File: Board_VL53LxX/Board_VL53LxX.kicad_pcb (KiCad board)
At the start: 2 copper layers, 20 x 16 mm, 11 parts, among them J1 Conn_01x06, U1 VL53L0X

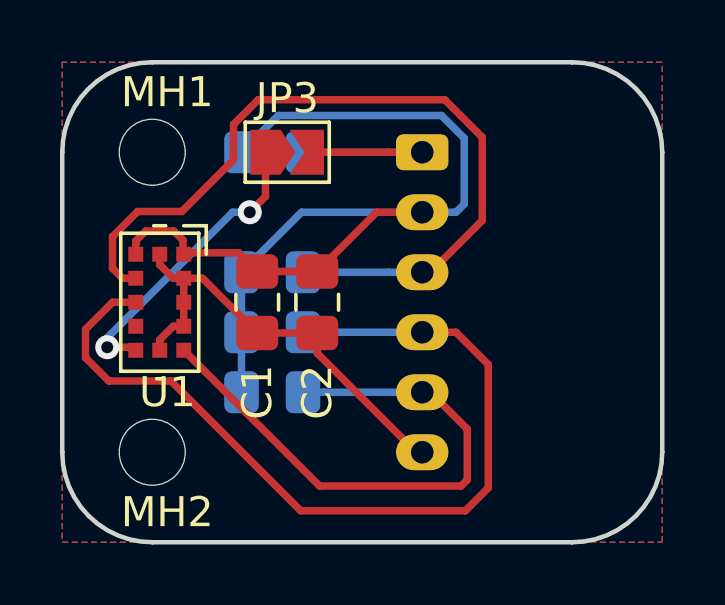
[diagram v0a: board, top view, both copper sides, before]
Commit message: update board
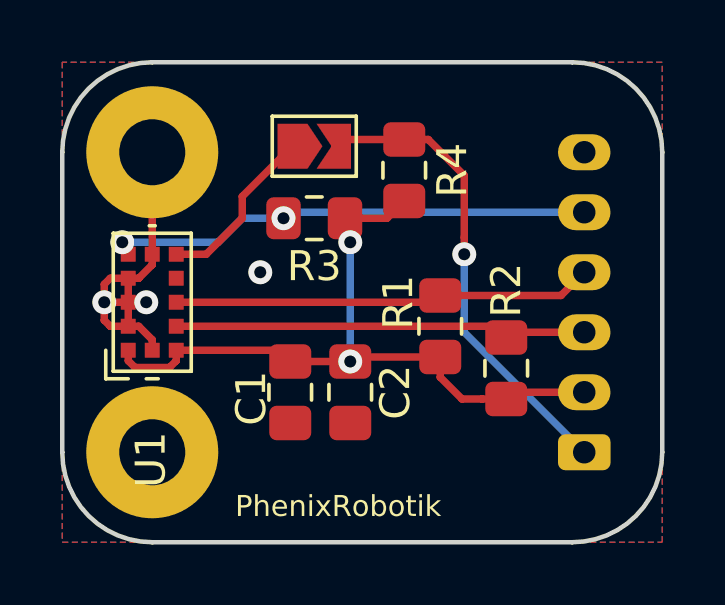
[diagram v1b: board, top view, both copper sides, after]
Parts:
- added LOGO1: Logo_Open_Hardware_Small, Symbol:OSHW-Logo2_7.3x6mm_SilkScreen, B.Cu at (107.6, 93.2)
- added LOGO2: Logo_Open_Hardware_Small, PhenixRobotik:Logo_8,5mm, B.Cu at (107.8, 84.4)
- MH1, MH2: value MountingHole -> MountingHole_Pad; footprint MountingHole:MountingHole_2.2mm_M2 -> MountingHole:MountingHole_2.2mm_M2_Pad
- R1, R2, R3, R4: moved to F.Cu
- U1: footprint PhoenixRobotik:TOF-12_4.4x2.4x1.0mm_P0.8mm -> PhenixRobotik:TOF-12_4.4x2.4x1.0mm_P0.8mm
- moved J1 11.4 mm to (117.4, 93.0), turned to 90 degrees
- moved R2 8.43 mm to (114.8, 90.2), turned to 90 degrees
- moved R3 5.97 mm to (108.4, 85.2), turned to 180 degrees
- moved R1 5.60 mm to (112.6, 88.8), turned to 270 degrees
- moved R4 4.44 mm to (111.4, 83.6), turned to 90 degrees
- moved C1 3.20 mm to (107.6, 91.0)
- moved C2 3.20 mm to (109.6, 91.0)
- moved JP3 0.92 mm to (108.4, 82.8)
- moved U1 0.25 mm to (103.0, 88.0), turned to 270 degrees
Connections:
- MH1 pad 1: (no net) -> GND
- MH2 pad 1: (no net) -> GND
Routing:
- net /I2C_SDA: track 29.6 -> 14.0 mm
- net /I2C_SCL: track 26.9 -> 14.1 mm
- net +2V8: track 34.6 -> 24.4 mm, vias 0 -> 2
- net /GPIO: track 7.75 -> 15.7 mm, vias 0 -> 1
- net Net-(JP3-Pad1): track 10.0 -> 5.79 mm, vias 2 -> 0
- net GND: track 15.0 -> 12.0 mm, vias 0 -> 2
- net /~XSHUT: track 19.1 -> 16.3 mm, vias 0 -> 2
- net (no net): vias 0 -> 1
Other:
- board text added: "PhenixRobotik"
